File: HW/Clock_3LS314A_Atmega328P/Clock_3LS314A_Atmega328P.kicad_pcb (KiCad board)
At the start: 4 copper layers, 41 x 23.5 mm, 50 parts, among them J1 Conn_02x02_Counter_Clockwise, J2 USB_C_Receptacle_PowerOnly_6P, J3 AVR_ISP, Q1 BC846, Q2 IRLML5203, Q3 2N7002, Q4 2N7002, Q5 2N7002, Q6 2N7002, SW1 CK_KMS2xxG, U1 ATmega328P-MM, U2 TP4056-42-ESOP8, U3 DW01A, U4 FS8205A, U5 74LVC1G125, Y1 SJK-7R-32.768-12.5-20-70-C

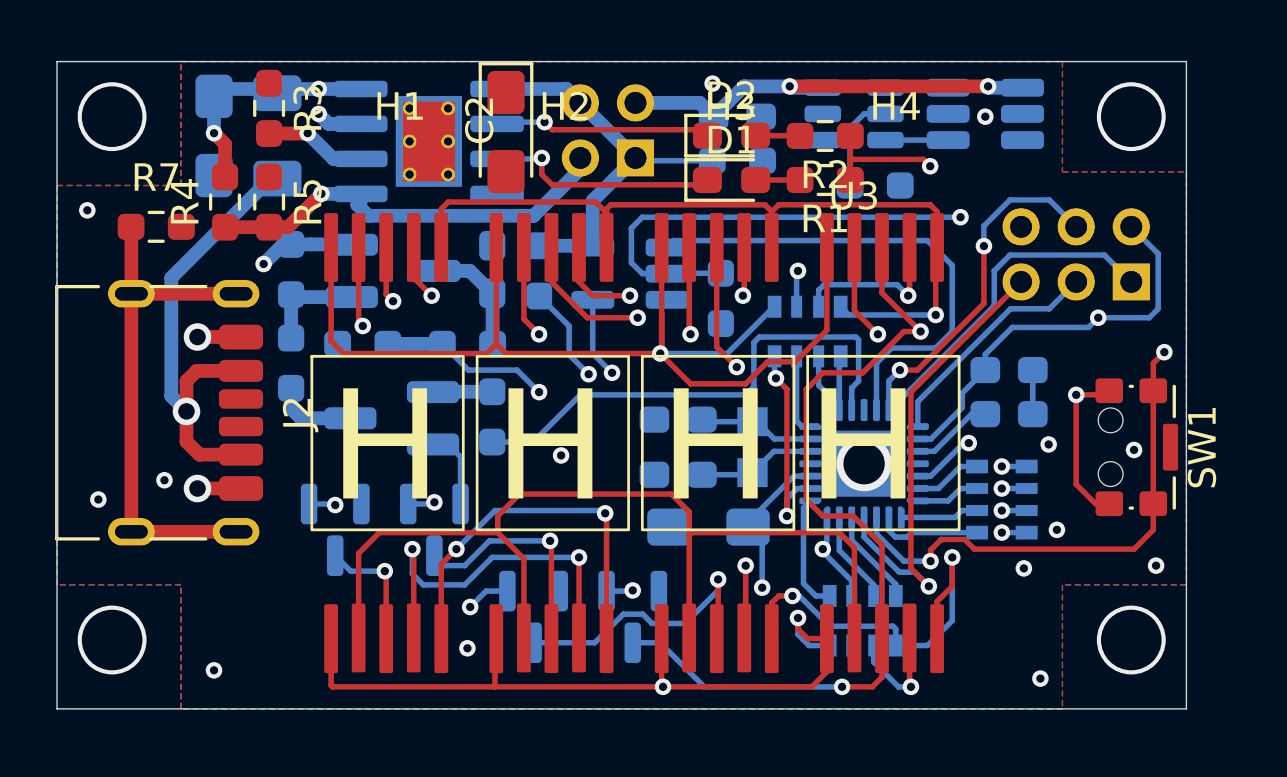
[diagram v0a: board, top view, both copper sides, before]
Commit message: pcb edit
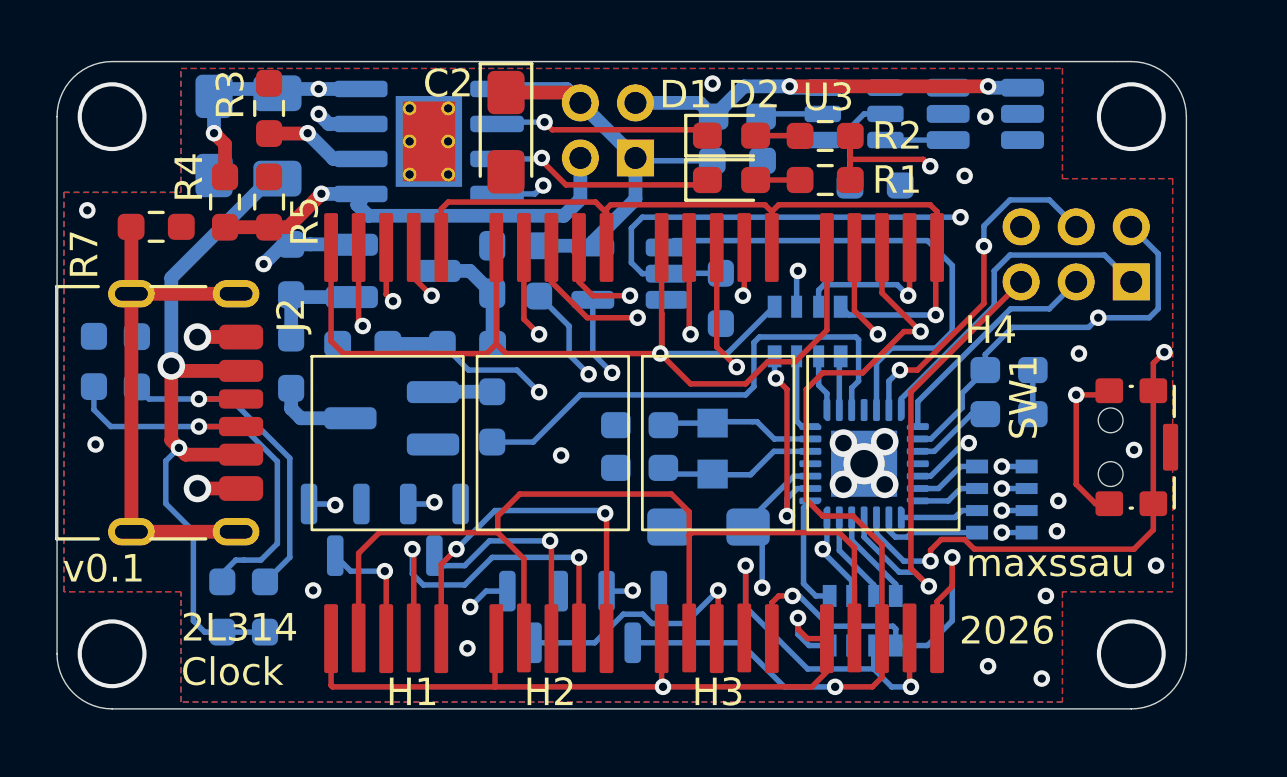
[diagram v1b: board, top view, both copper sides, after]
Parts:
- added R17: 10k, Resistor_SMD:R_0603_1608Metric_Pad0.98x0.95mm_HandSolder, B.Cu at (91.8, -42.1)
- added R18: 10k, Resistor_SMD:R_0603_1608Metric_Pad0.98x0.95mm_HandSolder, B.Cu at (93.4, -42.1)
- added R19: 10k, Resistor_SMD:R_0603_1608Metric_Pad0.98x0.95mm_HandSolder, B.Cu at (96.5, -33.2)
- added R20: 10k, Resistor_SMD:R_0603_1608Metric_Pad0.98x0.95mm_HandSolder, B.Cu at (98.0, -33.2)
- moved Y1 1.45 mm to (114.3, -39.0)
- moved C8 1.42 mm to (111.7, -38.2)
- moved C9 1.41 mm to (111.7, -39.8)
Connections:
- C1 pad 1: Net-(U2-V_{CC}) -> Net-(U2-CE)
- J2 pad A5: unconnected-(J2-CC1-PadA5) -> Net-(J2-CC1)
- J2 pad B5: unconnected-(J2-CC2-PadB5) -> Net-(J2-CC2)
- R1 pad 1: Net-(U2-V_{CC}) -> Net-(U2-CE)
- R2 pad 1: Net-(U2-V_{CC}) -> Net-(U2-CE)
- R4 pad 2: Net-(U2-V_{CC}) -> Net-(U2-CE)
- R6 pad 2: Net-(U2-V_{CC}) -> Net-(U2-CE)
- U2 pad 4: Net-(U2-V_{CC}) -> Net-(U2-CE)
- U2 pad 8: unconnected-(U2-CE-Pad8) -> Net-(U2-CE)
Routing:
- net Net-(U2-CE): track 0.00 -> 41.3 mm, vias 0 -> 4
- net Net-(U2-V_{CC}): track 36.8 -> 0.00 mm, vias 3 -> 0
- net /MCU/LED_SegC: track 20.5 -> 39.6 mm
- net Net-(J2-CC2): track 0.00 -> 15.7 mm, vias 0 -> 1
- net Net-(J2-CC1): track 0.00 -> 13.3 mm, vias 0 -> 1
- net /MCU/LED_SegDot: track 29.0 -> 38.3 mm
- net Net-(J2-VBUS-PadA9): track 16.9 -> 26.3 mm, vias 1 -> 2
- net Net-(U3-VCC): track 0.00 -> 3.90 mm
- net /MCU/MCU_VDD: track 38.9 -> 41.8 mm, vias 17 -> 11
- net /MCU/MCU_GND: track 12.8 -> 10.2 mm, vias 4 -> 16
- net Net-(U1-XTAL1/PB6): track 4.29 -> 6.17 mm
- net Net-(U1-XTAL2/PB7): track 4.23 -> 6.06 mm
- net Net-(J1-Pin_3): track 15.2 -> 15.9 mm
- net /MCU/MCU_VBAT_CONTROL: track 37.8 -> 37.3 mm
- added copper zone on In1.Cu, net /MCU/MCU_GND
- removed copper zone on In2.Cu, net /MCU/MCU_VDD
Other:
- outline, holes or cut-outs redrawn
- board text added: "2026"
- board text added: "2L314 Clock"
- board text added: "maxssau"
- board text added: "v0.1"
